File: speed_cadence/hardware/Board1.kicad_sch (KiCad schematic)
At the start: 17 parts, among them IC1 AH1912-W-7, J1 DX07S016JA3R1500, J2 Conn_01x04_Pin, J3 Conn_ST_STDC14, SW1 SW_Push, U1 STM32F042G6U6TR, U2 TS2940CW33_RPG, U4 TJA1051T-3

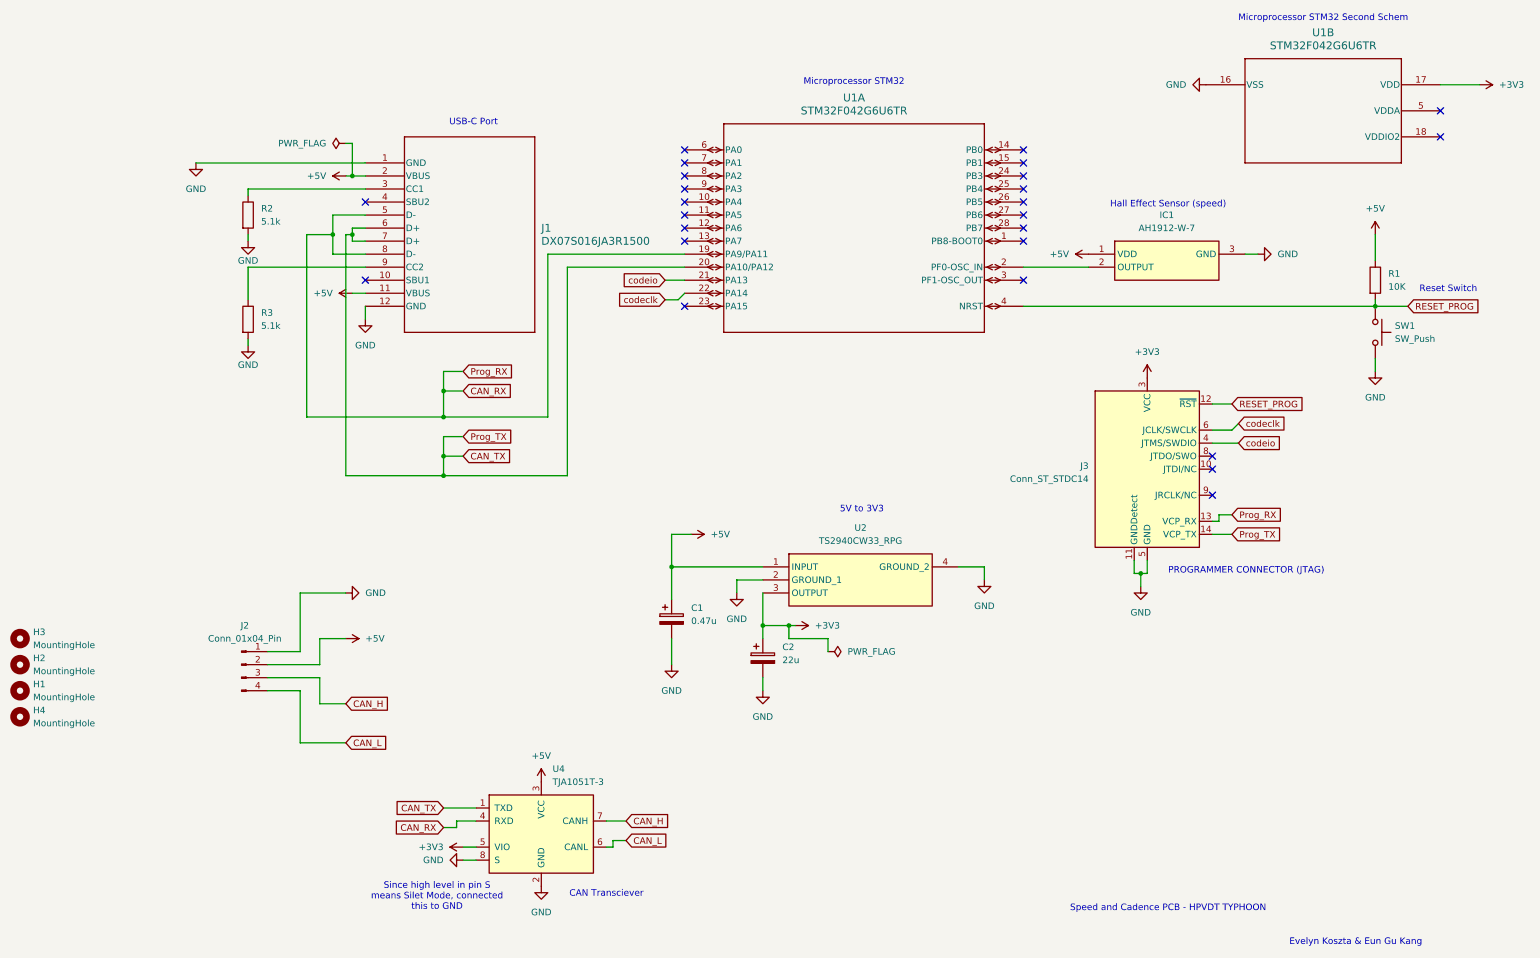
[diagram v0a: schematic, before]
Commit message: Updated board
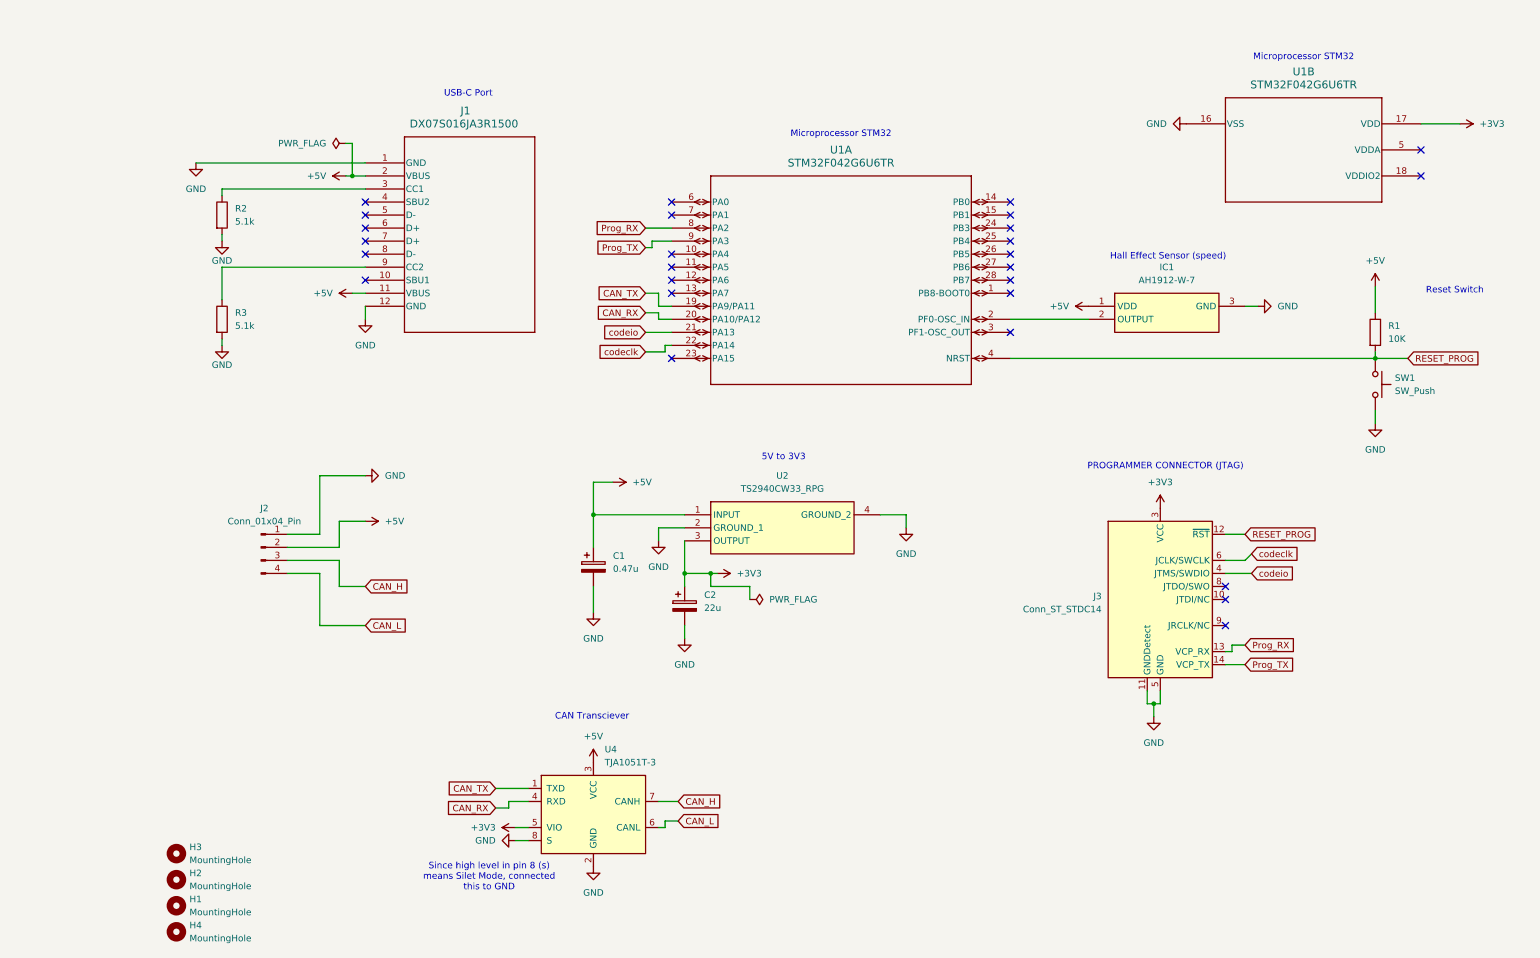
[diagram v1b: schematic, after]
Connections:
- net CAN_RX: now also U1.20 (PA10/PA12); no longer J1.5 (D-), J1.8 (D-), J3.13 (VCP_RX), U1.19 (PA9/PA11)
- net CAN_TX: now also U1.19 (PA9/PA11); no longer J1.6 (D+), J1.7 (D+), J3.14 (VCP_TX), U1.20 (PA10/PA12)
- net Prog_RX: now reaches U1.8 (PA2)
- net Prog_RX: now also J3.13 (VCP_RX)
- net Prog_TX: now reaches U1.9 (PA3)
- net Prog_TX: now also J3.14 (VCP_TX)
- no-connect marks 25 -> 27
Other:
- note added: "Since high level in pin 8 (s) means Silet Mode, connected this to GND"
- note removed: "Evelyn Koszta & Eun Gu Kang"
- note removed: "Microprocessor STM32 Second Schem"
- note removed: "Since high level in pin S means Silet Mode, connected this to GND"
- note removed: "Speed and Cadence PCB - HPVDT TYPHOON"
- company: (none) -> By Evelyn Koszta and Eun Gu Kang
- title: (none) -> Speed Measurement Board
- moved on the sheet: C1, C2, H1, H2, H3, H4, IC1, J2, J3, R1, R2, R3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
